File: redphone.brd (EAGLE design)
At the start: 139 x 65 mm, 247 parts, among them IC1 EP4CE15E22, IC10 74LVC1G02DCK, IC11 74LVC1G02DCK, IC12 74LVC1G02DCK, IC13 MAX1708, IC15 LSM303DLHC, IC16 EPCS4SI8N, IC17 L3GD20, IC18 WM8903, IC19 AT25SF041, IC2 STM32F429ZIT, IC20 MP34DT01, IC21 PT4181, IC22 MAX8903A, IC23 NRF24L01+, IC24 BME280, IC25 APDS-9960, IC3 MT48LC16M16A2TG, IC4 MAX8815A, IC5 TPS73025DBVT, IC6 LP3990MF-1.2, IC7 TPS63000, IC8 ESP8266, IC9 SIM800C, Q1 IRLML6402, Q10 NTA4153NT1G, Q2 NTA4153NT1G, Q4 NTA4153NT1G, Q6 IRLML6402, Q7 16MHz, Q8 NTA4153NT1G, SW1 PWR, SW2 CAM, SW3 VOL+, SW4 VOL-, X1 MICROSIM, X10 AUDIO-JACKSMD, X13 OV2640, X14 EXT, X15 DF13-4P-1.25V, X2 BAT, X3 RM68120_LCD, X7 CTS, Y1 2.4Ghz, Y3 2.4Ghz, Y4 GSM_PCB, Y5 2.4Ghz

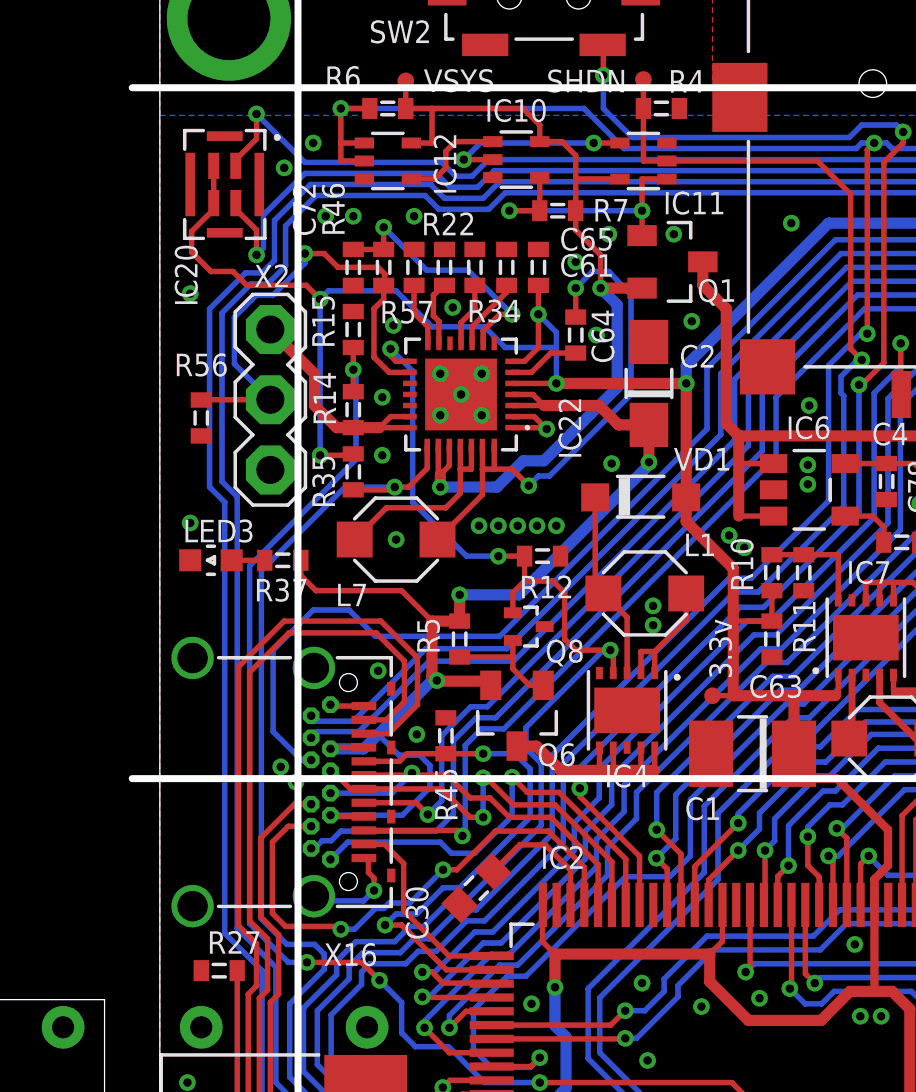
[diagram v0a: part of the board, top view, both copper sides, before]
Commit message: fix charger schematic
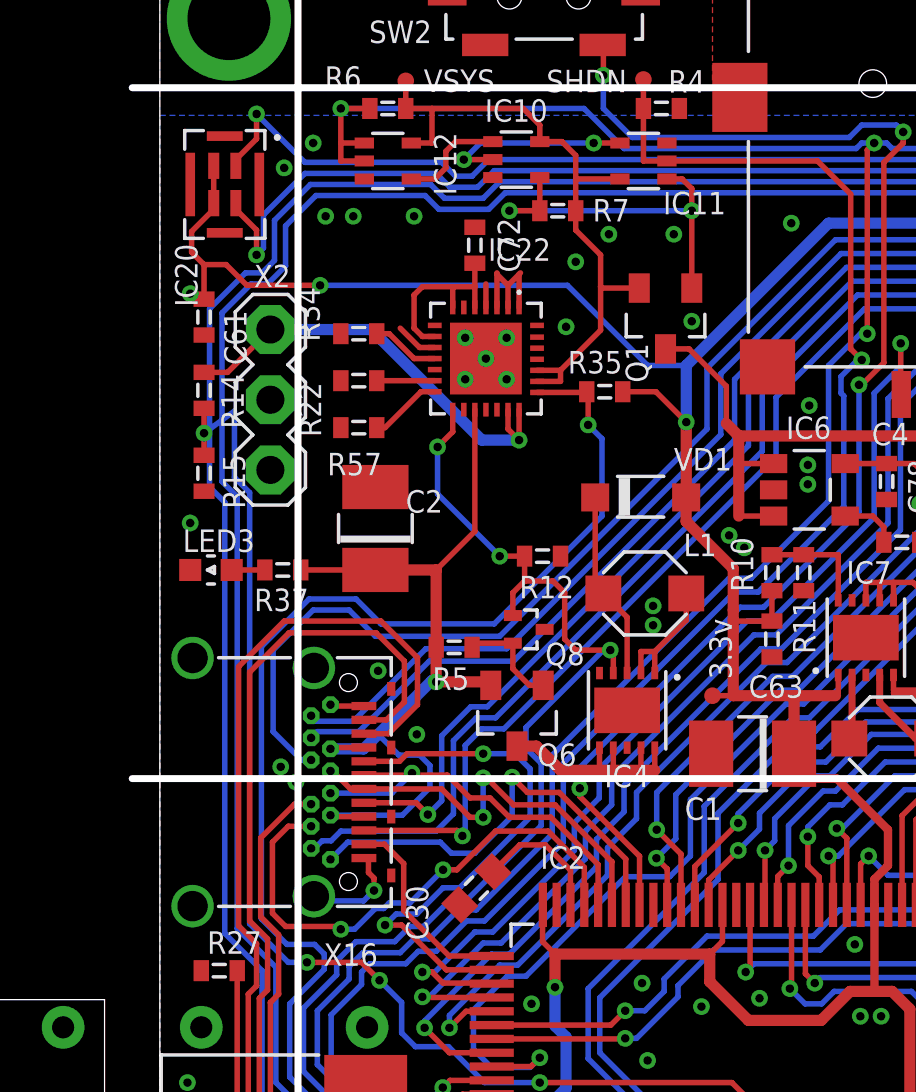
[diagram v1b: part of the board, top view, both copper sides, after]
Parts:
- removed C64, C65: 100n, netcat:R0402
- removed L7: 2.2uH, netcat:CDRH2D18LD
- removed R45, R46, R56: 10k, netcat:R0402
- C2: device netcat:SMC_A -> netcat:SMC_B
- moved C61 12.2 mm to (1.60, 49.7), turned to 270 degrees
- moved C2 11.2 mm to (7.80, 42.0)
- moved R35 9.55 mm to (16.1, 47.0), turned to 180 degrees
- moved R15 7.50 mm to (1.60, 44.0), turned to 90 degrees
- moved R57 6.14 mm to (7.20, 45.7), turned to 180 degrees
- moved R14 5.45 mm to (1.60, 47.0), turned to 90 degrees
- moved R22 5.14 mm to (7.20, 47.4), turned to 0 degrees
- moved R34 4.84 mm to (7.20, 49.1), turned to 0 degrees
- moved C72 4.47 mm to (11.4, 52.3), turned to 270 degrees
- moved Q1 2.07 mm to (18.3, 49.6), turned to 180 degrees
- moved IC22 1.58 mm to (11.8, 48.2), turned to 270 degrees
- moved R5 0.36 mm to (10.7, 37.8), turned to 0 degrees
- moved LED3 0.35 mm to (1.85, 40.5)
- moved R37 0.35 mm to (4.45, 40.5)
- moved Q8 0.10 mm to (13.3, 38.4)
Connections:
- removed net N$10: C64.1, IC22.6
- removed net N$28: IC22.25, IC22.26, L7.2
- removed net N$61: C65.1, IC22.10
- removed net N$87: IC22.16, R46.1, R56.1, X2.2
- removed net N$88: C72.2, IC22.9, R46.2
- net 3.3V: no longer IC22.5, IC22.7
- net GND: now also IC22.10, IC22.16, IC22.3, IC22.4; no longer C65.2, IC22.17, R45.1, R56.2
- net N$6: now also C72.2, IC22.5, IC22.7, IC22.9; no longer C64.2, IC22.27, IC22.28, L7.1
- net USB_CC1: no longer R45.2
- net V_USB: now also IC22.17; no longer IC22.3, IC22.4
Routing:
- net N$87: track 17.6 -> 0.00 mm, vias 1 -> 0
- net N$6: track 19.2 -> 6.75 mm, vias 2 -> 0
- net V_USB: track 43.7 -> 31.9 mm, vias 3 -> 1
- net 3.3V: track 787.1 -> 776.5 mm, vias 53 -> 50
- net N$88: track 9.60 -> 0.00 mm, vias 2 -> 0
- net BAT_CHG: track 41.8 -> 50.7 mm
- net V_SYS: track 33.0 -> 24.1 mm, vias 2 -> 0
- net V_BAT: track 8.51 -> 16.1 mm, vias 0 -> 1
- net N$28: track 7.49 -> 0.00 mm
- net PWR_OTG_MODE: track 52.4 -> 48.1 mm
- net GND: track 34.4 -> 38.6 mm, vias 450 -> 438
- net BAT_EN: track 10.1 -> 13.5 mm
- net N$61: track 2.62 -> 0.00 mm
- net N$10: track 2.59 -> 0.00 mm
- net V_INT: track 61.5 -> 59.4 mm
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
